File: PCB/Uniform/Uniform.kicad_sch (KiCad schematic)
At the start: 156 parts, among them CON1 826629-5, CON2 Conn_01x03, U1 STM32L072KZT6

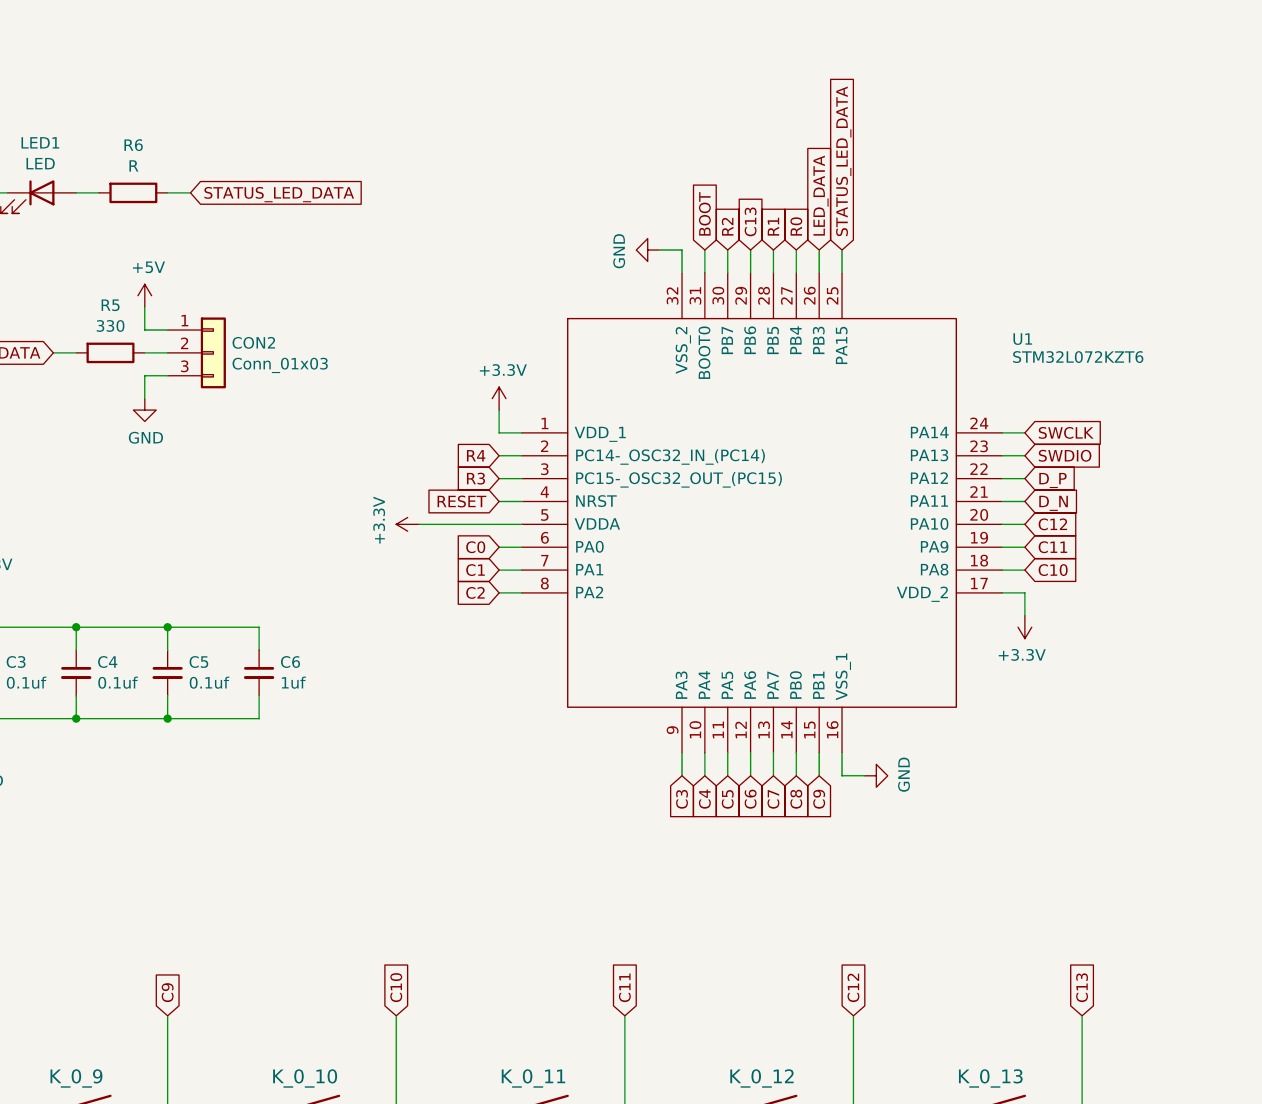
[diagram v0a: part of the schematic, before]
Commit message: Moved mount holes so the drill points in the plate won't collide with switch clip-in points
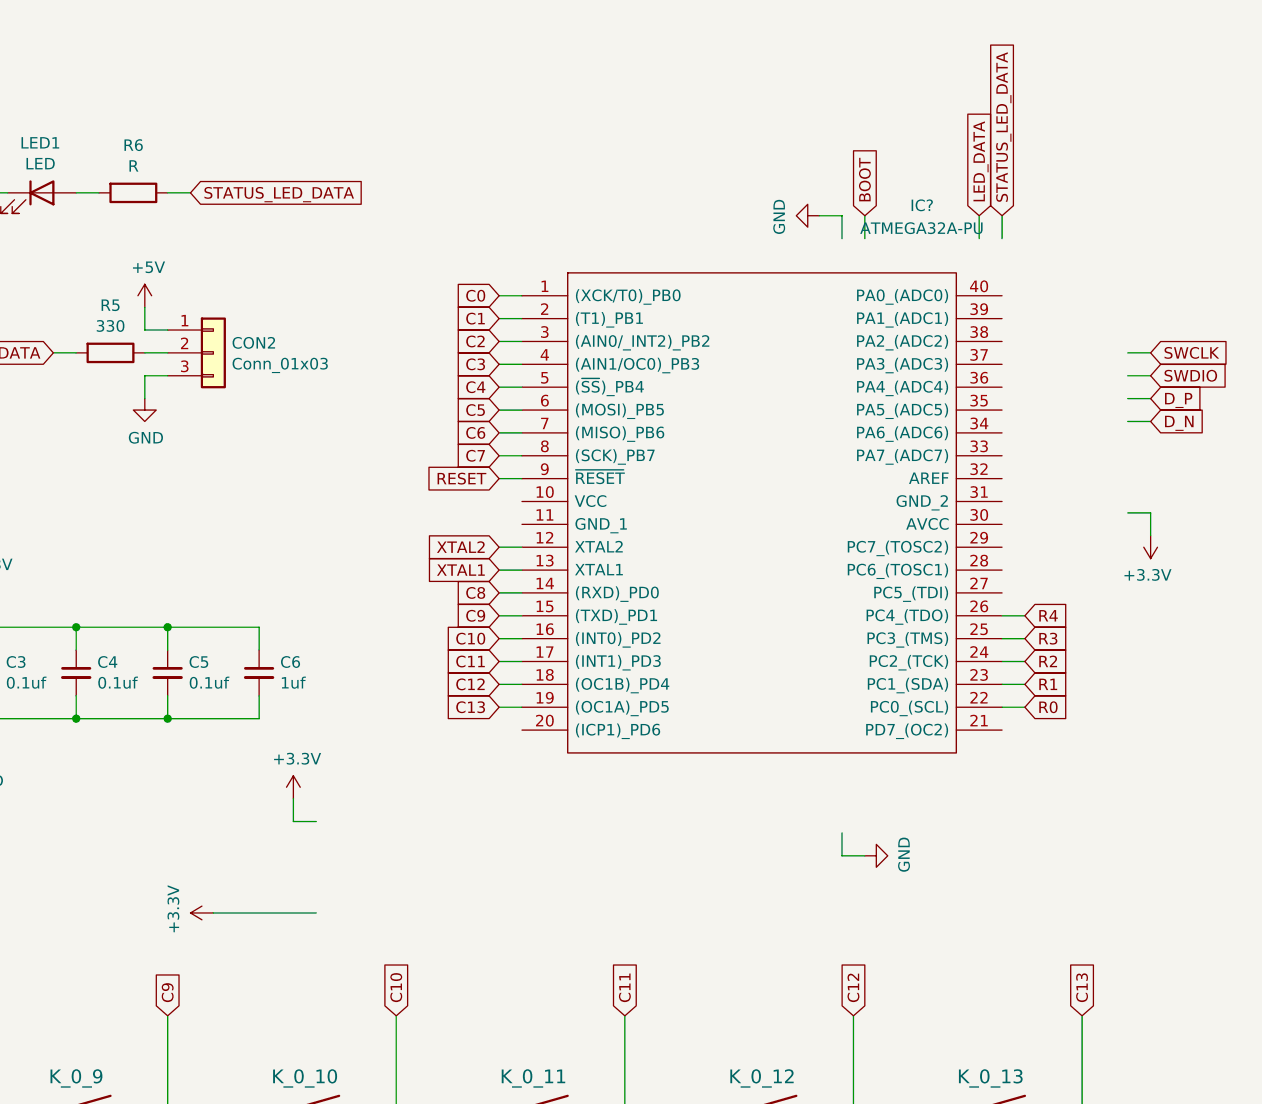
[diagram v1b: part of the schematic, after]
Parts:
- removed U1: STM32L072KZT6, STM32L072KZT6:QFP80P900X900X160-32N, symbol STM32L072KZT6:STM32L072KZT6
- added IC?: ATMEGA32A-PU, DIP1556W56P254L5232H483Q40N, symbol ATMEGA32A-PU:ATMEGA32A-PU
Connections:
- net C0: now also IC?.1 ((XCK/T0)_PB0)
- net C1: now also IC?.2 ((T1)_PB1)
- net C10: now also IC?.16 ((INT0)_PD2)
- net C11: now also IC?.17 ((INT1)_PD3)
- net C12: now also IC?.18 ((OC1B)_PD4)
- net C13: now also IC?.19 ((OC1A)_PD5)
- net C2: now also IC?.3 ((AIN0/_INT2)_PB2)
- net C3: now also IC?.4 ((AIN1/OC0)_PB3)
- net C4: now also IC?.5 ((~{SS})_PB4)
- net C5: now also IC?.6 ((MOSI)_PB5)
- net C6: now also IC?.7 ((MISO)_PB6)
- net C7: now also IC?.8 ((SCK)_PB7)
- net C8: now also IC?.14 ((RXD)_PD0)
- net C9: now also IC?.15 ((TXD)_PD1)
- net R0: now also IC?.22 (PC0_(SCL))
- net R1: now also IC?.23 (PC1_(SDA))
- net R2: now also IC?.24 (PC2_(TCK))
- net R3: now also IC?.25 (PC3_(TMS))
- net R4: now also IC?.26 (PC4_(TDO))
- net RESET: now also IC?.9 (~{RESET})
- new net XTAL1: IC?.13 (XTAL1)
- new net XTAL2: IC?.12 (XTAL2)

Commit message: revert ATMEGA32 changes to schematic that were lumped into last commit
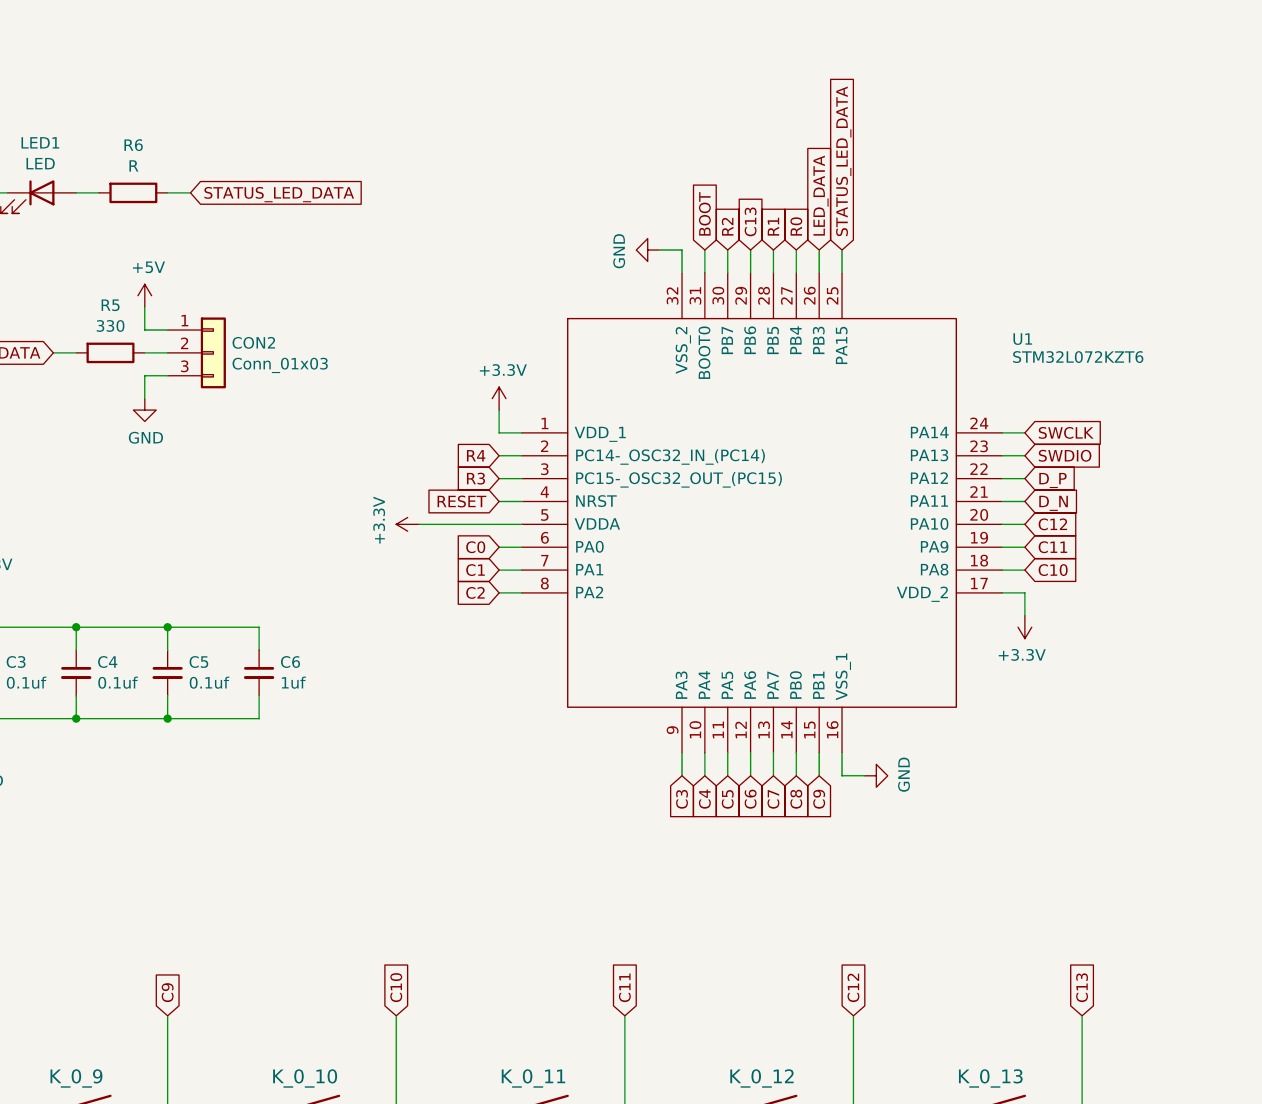
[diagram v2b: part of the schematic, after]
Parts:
- removed IC?: ATMEGA32A-PU, DIP1556W56P254L5232H483Q40N, symbol ATMEGA32A-PU:ATMEGA32A-PU
- added U1: STM32L072KZT6, STM32L072KZT6:QFP80P900X900X160-32N, symbol STM32L072KZT6:STM32L072KZT6
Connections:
- net +3V3: now also U1.1 (VDD_1), U1.17 (VDD_2), U1.5 (VDDA)
- net BOOT: now also U1.31 (BOOT0)
- net C0: now also U1.6 (PA0)
- net C1: now also U1.7 (PA1)
- net C10: now also U1.18 (PA8)
- net C11: now also U1.19 (PA9)
- net C12: now also U1.20 (PA10)
- net C13: now also U1.29 (PB6)
- net C2: now also U1.8 (PA2)
- net C3: now also U1.9 (PA3)
- net C4: now also U1.10 (PA4)
- net C5: now also U1.11 (PA5)
- net C6: now also U1.12 (PA6)
- net C7: now also U1.13 (PA7)
- net C8: now also U1.14 (PB0)
- net C9: now also U1.15 (PB1)
- net D_N: now also U1.21 (PA11)
- net D_P: now also U1.22 (PA12)
- net GND: now also U1.16 (VSS_1), U1.32 (VSS_2)
- net LED_DATA: now also U1.26 (PB3)
- net R0: now also U1.27 (PB4)
- net R1: now also U1.28 (PB5)
- net R2: now also U1.30 (PB7)
- net R3: now also U1.3 (PC15-_OSC32_OUT_(PC15))
- net R4: now also U1.2 (PC14-_OSC32_IN_(PC14))
- net RESET: now also U1.4 (NRST)
- net STATUS_LED_DATA: now also U1.25 (PA15)
- net SWCLK: now also U1.24 (PA14)
- net SWDIO: now also U1.23 (PA13)
